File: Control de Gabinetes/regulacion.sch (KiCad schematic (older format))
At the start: 13 parts, among them J1 Conn_01x03_MountingPin, U2 LM1117-3.3, U3 LM1117-5.0

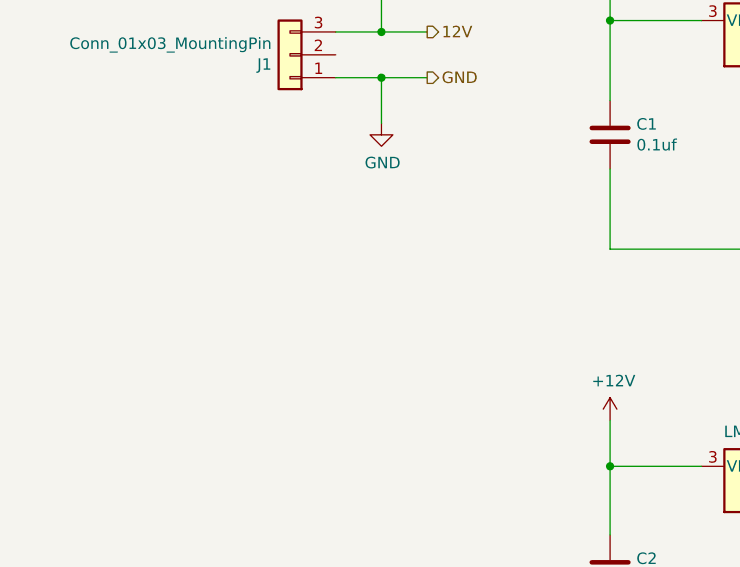
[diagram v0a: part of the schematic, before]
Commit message: avance 20/07/2021
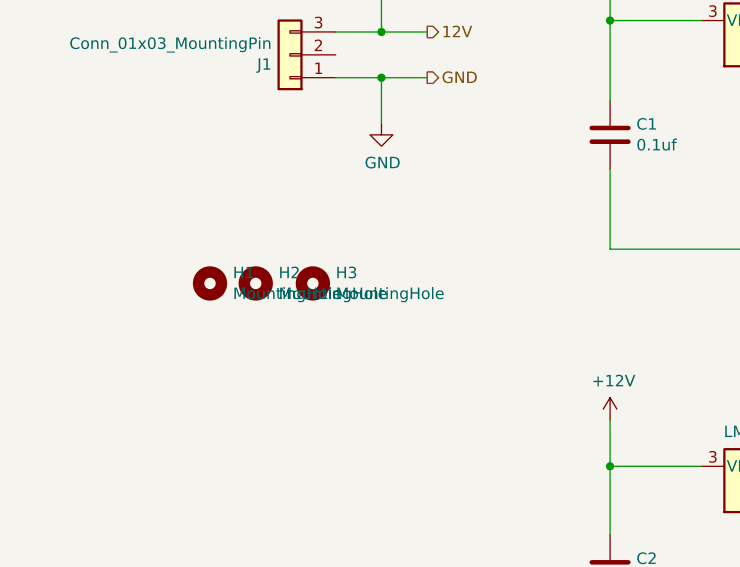
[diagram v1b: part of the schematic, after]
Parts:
- added H1, H2, H3: MountingHole, MountingHole:MountingHole_3.5mm, symbol Mechanical:MountingHole
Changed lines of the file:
@@
 	5000 4300 4300 4300
 Connection ~ 4300 4300
+$Comp
+L Mechanical:MountingHole H2
+U 1 1 610E1A2D
+P 1550 2500
+F 0 "H2" H 1650 2546 50  0000 L CNN
+F 1 "MountingHole" H 1650 2455 50  0000 L CNN
+F 2 "MountingHole:MountingHole_3.5mm" H 1550 2500 50  0001 C CNN
+F 3 "~" H 1550 2500 50  0001 C CNN
+	1    1550 2500
+	1    0    0    -1
+$EndComp
+$Comp
+L Mechanical:MountingHole H1
+U 1 1 610E2A51
+P 1350 2500
+F 0 "H1" H 1450 2546 50  0000 L CNN
+F 1 "MountingHole" H 1450 2455 50  0000 L CNN
+F 2 "MountingHole:MountingHole_3.5mm" H 1350 2500 50  0001 C CNN
+F 3 "~" H 1350 2500 50  0001 C CNN
+	1    1350 2500
+	1    0    0    -1
+$EndComp
+$Comp
+L Mechanical:MountingHole H3
+U 1 1 610E2D5F
+P 1800 2500
+F 0 "H3" H 1900 2546 50  0000 L CNN
+F 1 "MountingHole" H 1900 2455 50  0000 L CNN
+F 2 "MountingHole:MountingHole_3.5mm" H 1800 2500 50  0001 C CNN
+F 3 "~" H 1800 2500 50  0001 C CNN
+	1    1800 2500
+	1    0    0    -1
+$EndComp
 $EndSCHEMATC
